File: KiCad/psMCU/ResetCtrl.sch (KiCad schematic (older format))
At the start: 16 parts

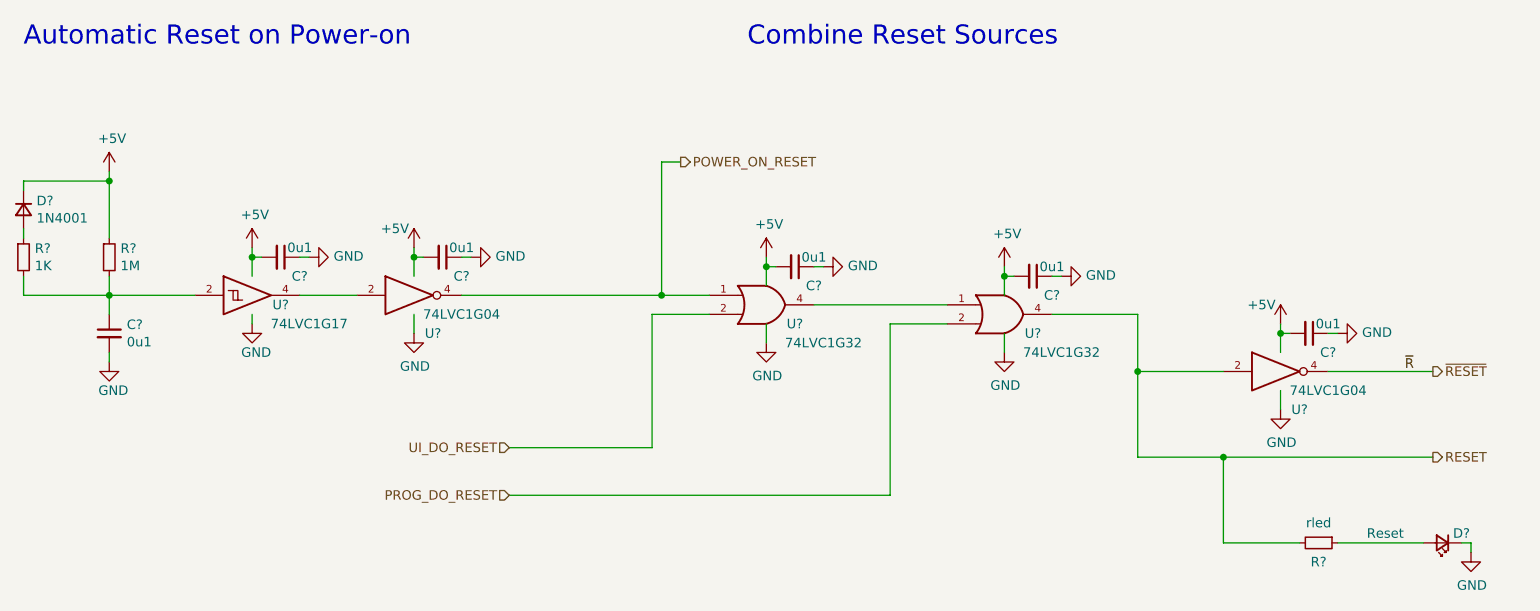
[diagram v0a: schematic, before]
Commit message: First Schematic Draft done.
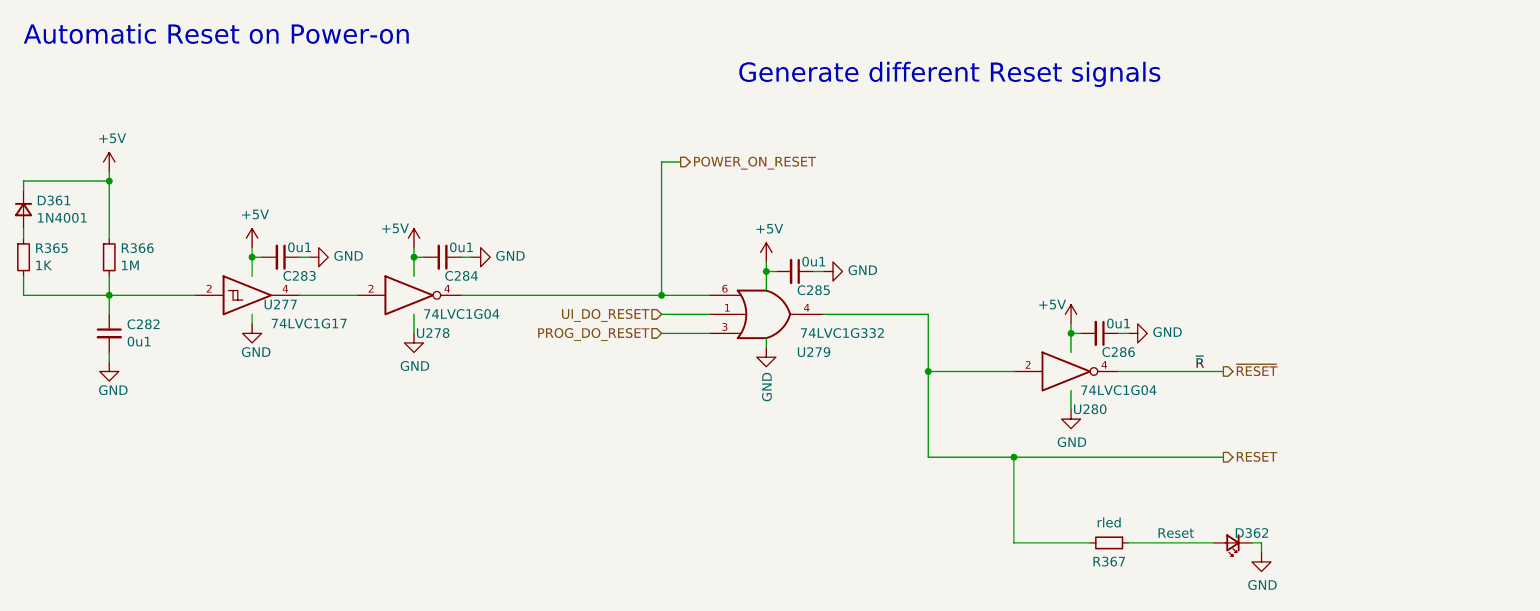
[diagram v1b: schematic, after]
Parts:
- removed C? (x2): 0u1, Capacitor_SMD:C_0603_1608Metric, symbol Device:C_Small
- removed U? (x2): 74LVC1G32, Package_TO_SOT_SMD:SOT-353_SC-70-5, symbol 74xGxx:74LVC1G32
- added C285: 0u1, NoRef_Footprints:C_0603_1608Metric_NoRef, symbol Device:C_Small
- added U279: 74LVC1G332, symbol 74xGxx:74LVC1G332
- C282, C283, C284, C286: renamed from C?; footprint Capacitor_SMD:C_0603_1608Metric -> NoRef_Footprints:C_0603_1608Metric_NoRef
- D362: renamed from D?; footprint Diode_SMD:D_0603_1608Metric -> NoRef_Footprints:D_0603_1608Metric_NoRef
- R367: renamed from R?; footprint Resistor_SMD:R_0603_1608Metric -> NoRef_Footprints:R_0603_1608Metric
- gave numbers to parts that had none: 6
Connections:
- net +5V: now also C285.2, U279.5 (VCC)
- net GND: now also C285.1, U279.2 (GND)
- net POWER_ON_RESET: now also U279.6
- net PROG_DO_RESET: now also U279.3
- net RESET: now also U279.4
- net UI_DO_RESET: now also U279.1
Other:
- note added: "Generate different Reset signals"
- note removed: "Combine Reset Sources"
- moved on the sheet: C286, D362, R367, U280
